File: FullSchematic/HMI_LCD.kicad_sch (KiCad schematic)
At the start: 31 parts, among them J10 LCD_Conn, J5 2x6 Pin Header, Q3 NPN, U10 SN74LVC2T45DCURE4, U11 SN74LVC2T45DCURE4, U12 SN74LVC2T45DCURE4, U13 SN74LVC2T45DCURE4, U14 SN74LV595ARGYR, U9 L79L05ABD13TR

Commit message: Semi-complete board
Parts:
- J5: footprint Connector_PinHeader_2.54mm:PinHeader_2x06_P2.54mm_Vertical -> CustomFootprints:PMOD
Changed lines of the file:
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@@
       (effects (font (size 1.27 1.27)))
     )
-    (property "Footprint" "Connector_PinHeader_2.54mm:PinHeader_2x06_P2.54mm_Vertical" (at 118.0592 51.816 0)
+    (property "Footprint" "CustomFootprints:PMOD" (at 118.0592 51.816 0)
       (effects (font (size 1.27 1.27)) (justify bottom) hide)
     )

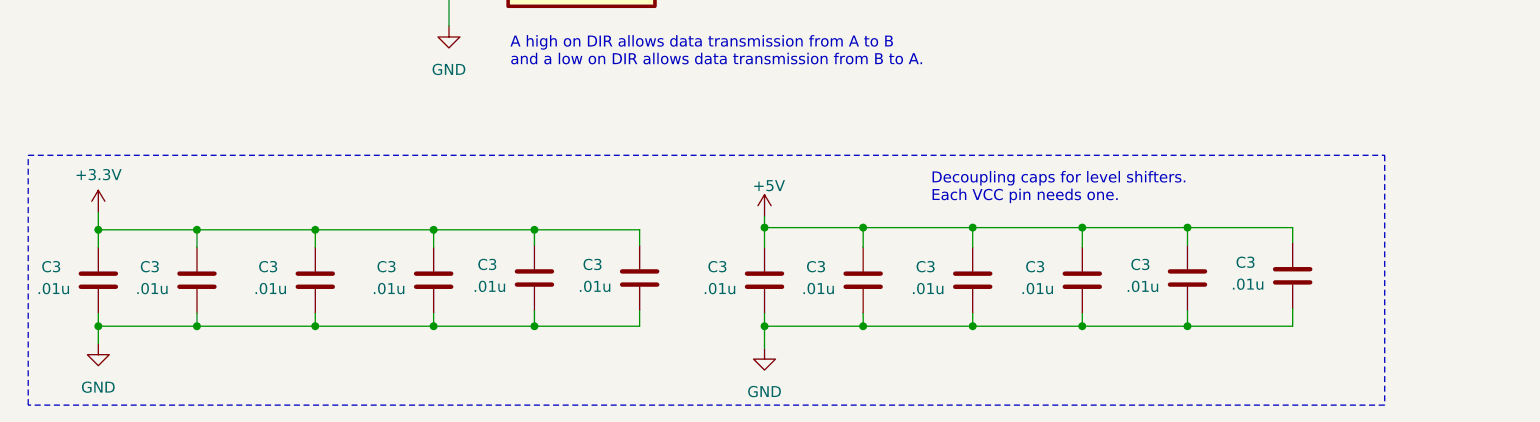
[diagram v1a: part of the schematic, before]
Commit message: PCB V.1
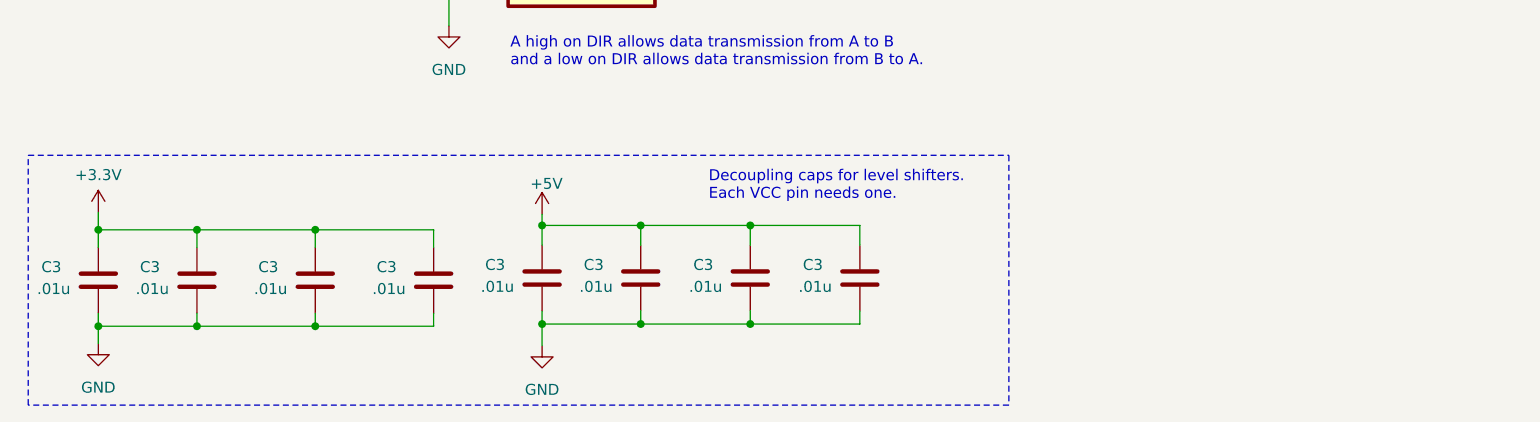
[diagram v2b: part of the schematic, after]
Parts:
- removed C3 (x4): .01u, Capacitor_SMD:C_0805_2012Metric, symbol Device:C
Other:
- moved on the sheet: C3
